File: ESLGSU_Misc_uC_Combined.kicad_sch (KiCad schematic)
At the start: 6 parts, among them U57 CY8C9520A, U74 PCAL6524HEAZ

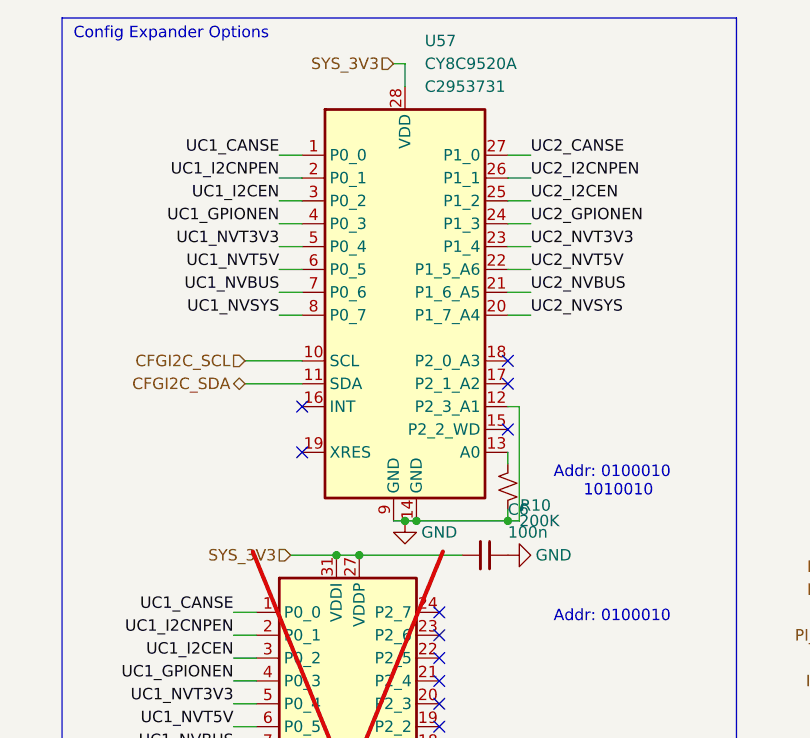
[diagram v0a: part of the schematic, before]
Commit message: Should be done with minimal version
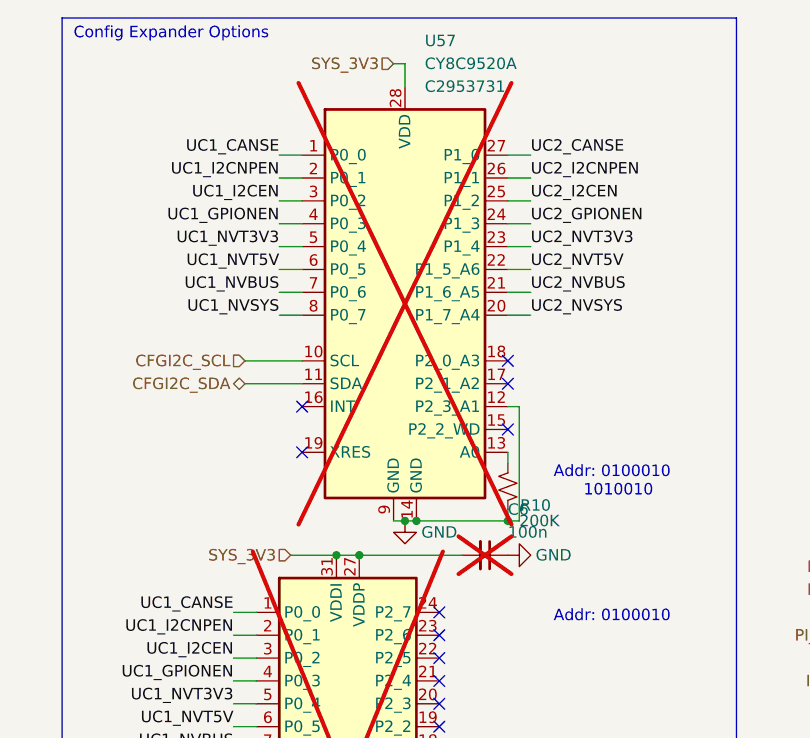
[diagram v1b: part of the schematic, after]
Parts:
- C6, U57: now not fitted; now left out of the parts list
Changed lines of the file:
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@@
   )
   (symbol (lib_id "Device:C_Small") (at 212.09 90.17 270) (unit 1)
-    (in_bom yes) (on_board yes) (dnp no)
+    (in_bom no) (on_board yes) (dnp yes)
     (property "Reference" "C6" (at 214.63 85.09 90)
       (effects (font (size 1.27 1.27)) (justify left))
@@
   )
   (symbol (lib_id "ESLGSU_Parts_Lib:CY8C9520A") (at 203.2 54.61 0) (unit 1)
-    (in_bom yes) (on_board yes) (dnp no) (fields_autoplaced)
+    (in_bom no) (on_board yes) (dnp yes) (fields_autoplaced)
     (property "Reference" "U57" (at 205.3941 33.02 0)
       (effects (font (size 1.27 1.27)) (justify left))
